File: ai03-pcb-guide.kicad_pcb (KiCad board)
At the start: 2 copper layers, 65.9 x 38.1 mm, 24 parts, among them SW1 SW_Push, U1 ATmega32U4-A, Y1 16Mhz

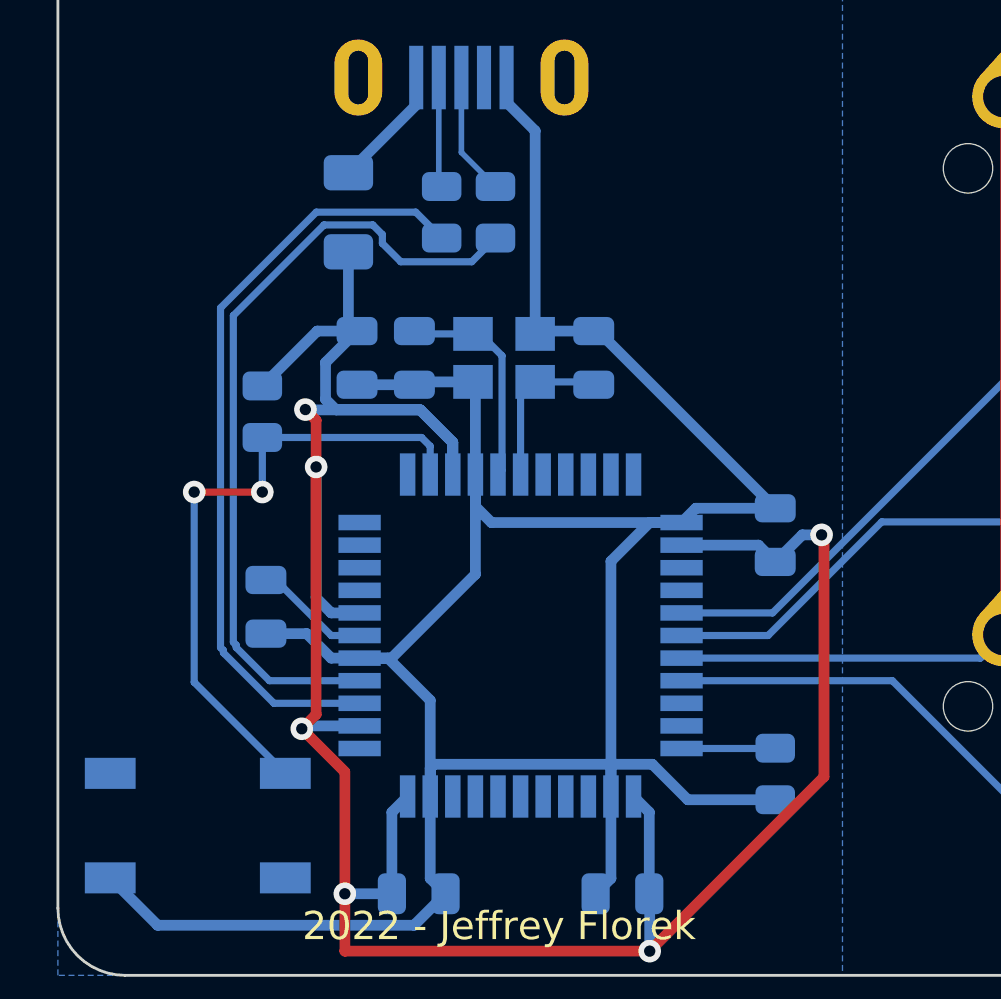
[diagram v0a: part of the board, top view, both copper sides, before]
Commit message: Add silly line art of my dog to the PCB.
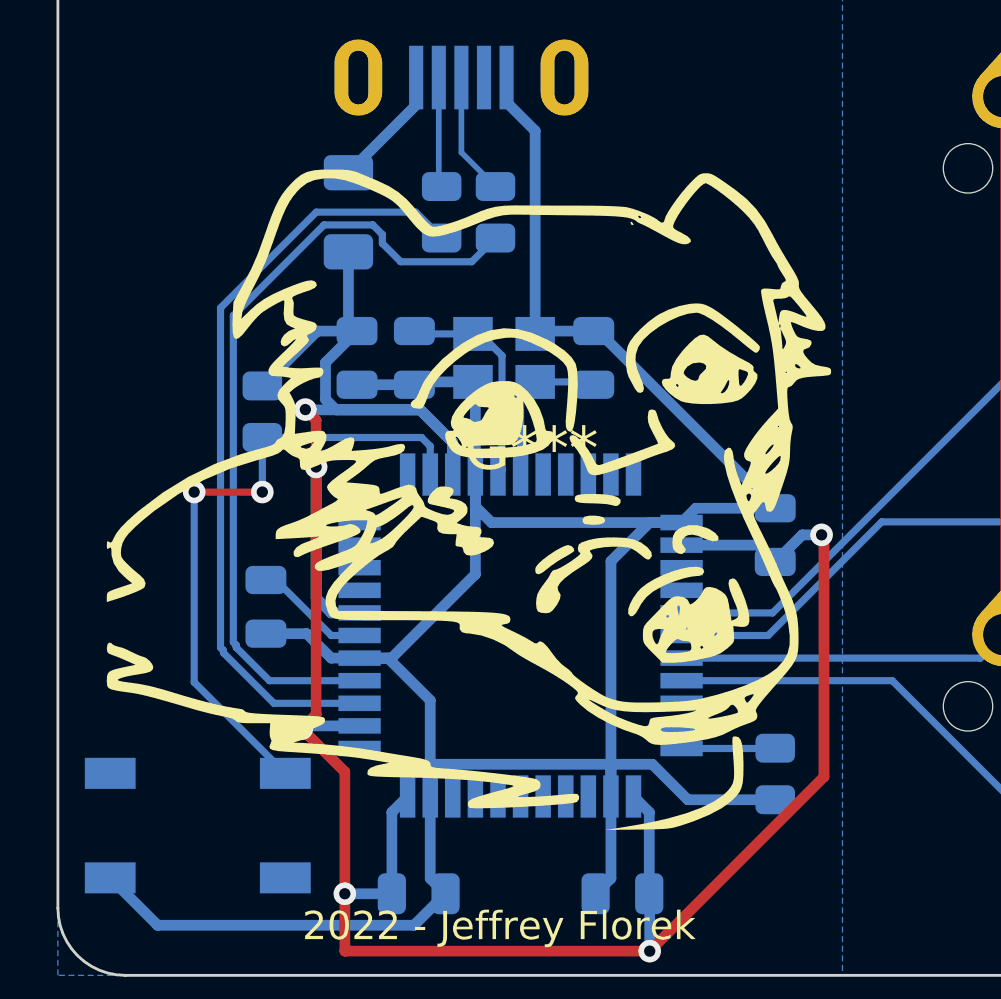
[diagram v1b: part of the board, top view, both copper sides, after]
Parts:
- added G***: LOGO, LOGO, F.Cu at (124.7, 107.6)
